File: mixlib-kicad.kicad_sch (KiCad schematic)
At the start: 15 parts, among them Q1 DMT6005LPS, Q2 STL130N6F7, U1 MCP6401, U2 MCP6401

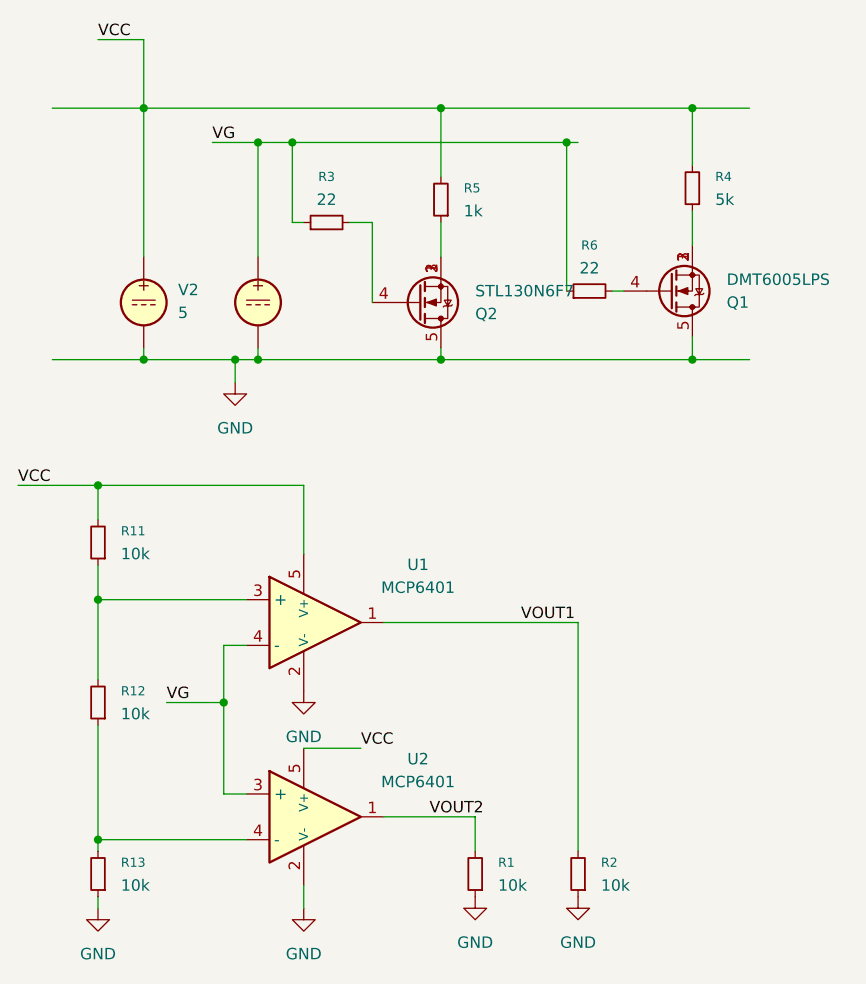
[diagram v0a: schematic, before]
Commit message: chore: saving project state
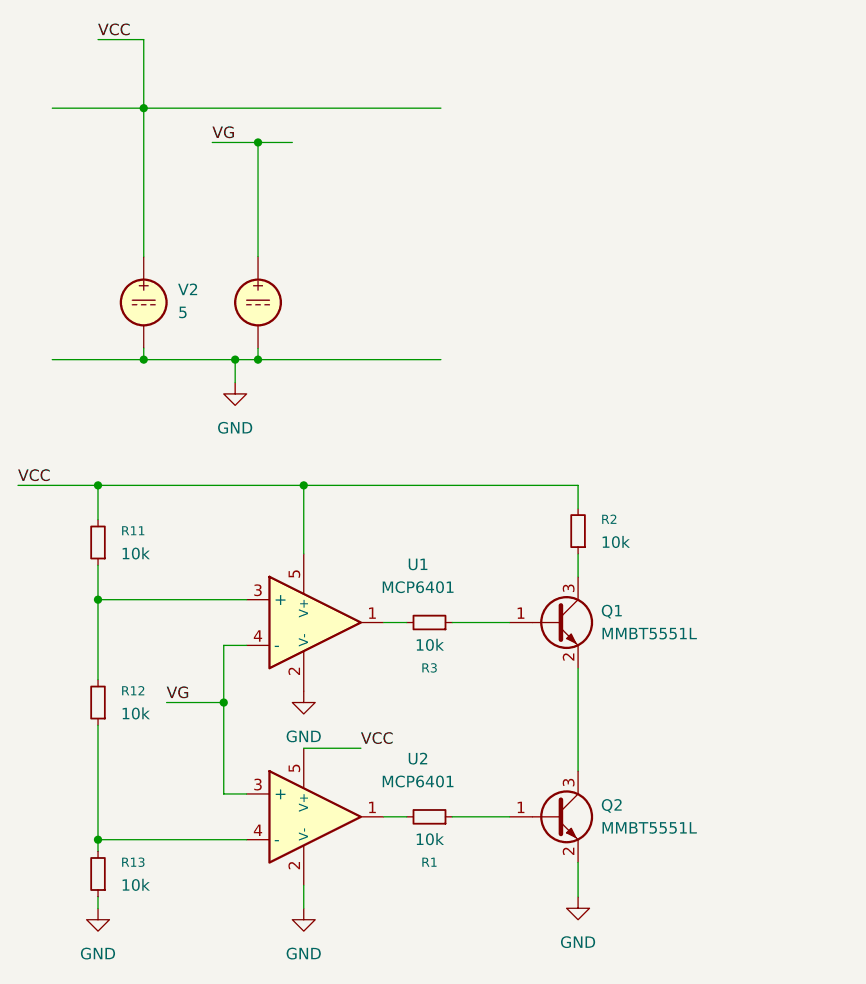
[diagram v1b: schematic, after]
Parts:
- removed Q1: DMT6005LPS, mixlib-discrete-mosfet:POWERDI5060-8, symbol mixlib-discrete-mosfet:DMT6005LPS
- removed Q2: STL130N6F7, mixlib-discrete-mosfet:POWERFLAT_5X6_C_STM, symbol mixlib-discrete-mosfet:STL130N6F7
- removed R4: 5k, symbol Device:R_Small
- removed R5: 1k, symbol Device:R_Small
- removed R6: 22, symbol Device:R_Small
- added Q1, Q2: MMBT5551L, Package_TO_SOT_SMD:SOT-23, symbol mixlib-discrete-npn:MMBT5551L
- R3: value 22 -> 10k
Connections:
- net GND: now also Q2.2 (E); no longer R1.1, R2.1
- net VCC: now also R2.2
- net VG: no longer R3.1
- net at R3.2: now also U1.1
- removed net VOUT1: R2.2, U1.1
- net VOUT2: no longer names the net of R1.2, U2.1
- new net: Q1.1 (B), R3.1
- new net: Q1.3 (C), R2.1
- new net: Q2.1 (B), R1.1
- new net: Q1.2 (E), Q2.3 (C)
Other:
- moved on the sheet: R1
